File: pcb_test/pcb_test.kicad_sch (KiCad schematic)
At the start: 1 part, among them U1 STM32U5G9ZJJxQ

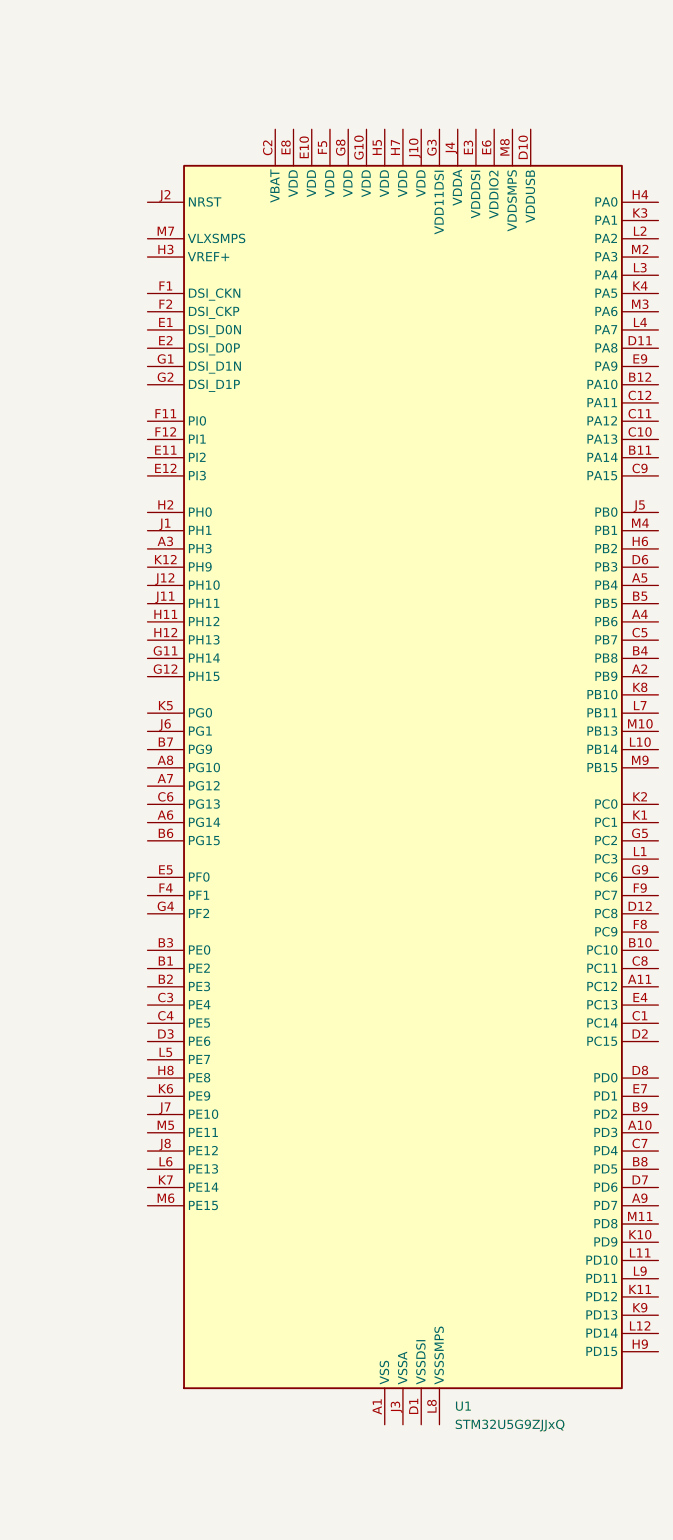
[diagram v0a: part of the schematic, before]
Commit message: Ajout testpoints
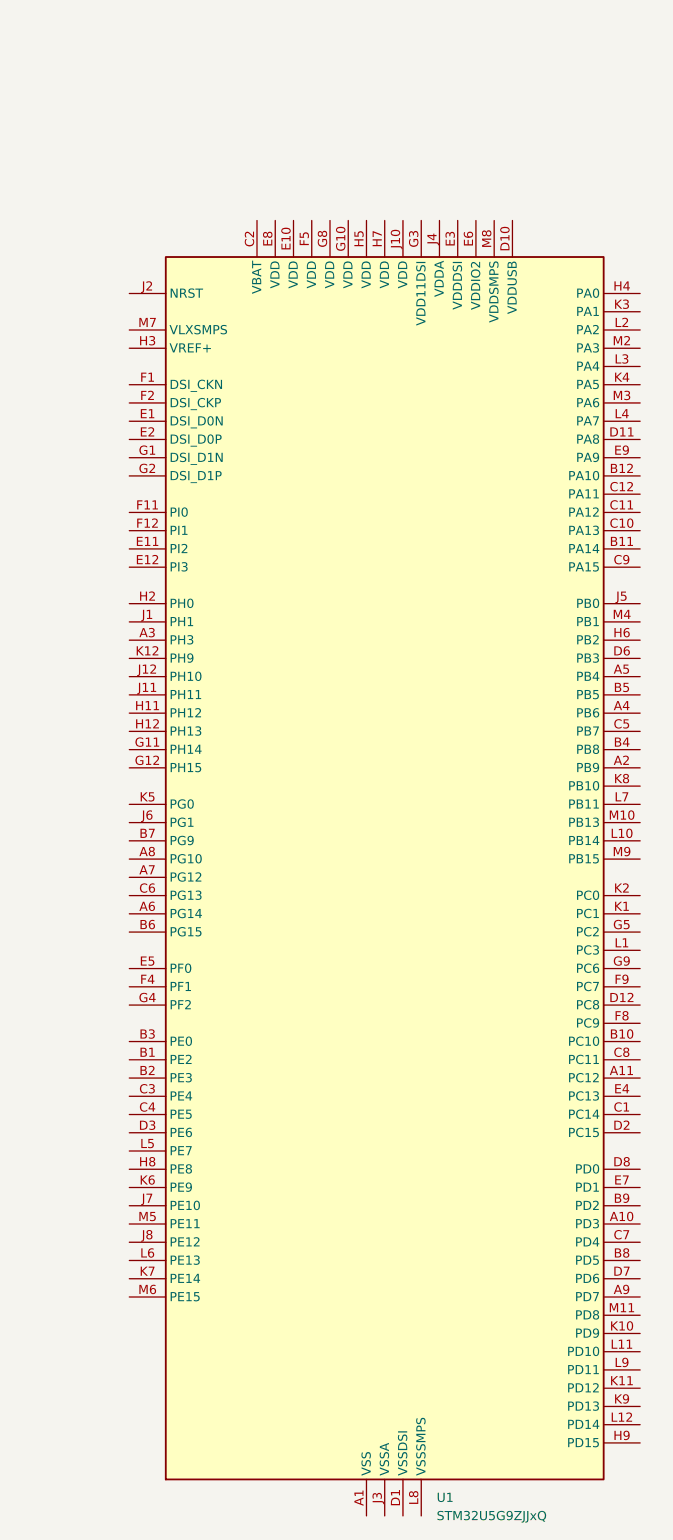
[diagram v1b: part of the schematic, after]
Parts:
- U1: footprint Package_BGA:UFBGA-144_10x10mm_Layout12x12_P0.8mm -> Package_QFP:LQFP-144_20x20mm_P0.5mm
